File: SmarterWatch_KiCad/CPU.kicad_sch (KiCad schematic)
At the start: 14 parts, among them SW1 SW_SPST, SW2 SW_SPST, U5 ESP32-C6-MINI-1

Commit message: Button Footprint
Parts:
- SW1, SW2: footprint Smarter watching stuff foot:Button_smd_spst -> Custom_Foot:SMD_Button_6mm_SPST
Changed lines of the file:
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@@
 			)
 		)
-		(property "Footprint" "Smarter watching stuff foot:Button_smd_spst"
+		(property "Footprint" "Custom_Foot:SMD_Button_6mm_SPST"
 			(at 101.6 110.49 0)
 			(effects
@@
 			)
 		)
-		(property "Footprint" "Smarter watching stuff foot:Button_smd_spst"
+		(property "Footprint" "Custom_Foot:SMD_Button_6mm_SPST"
 			(at 82.55 81.28 0)
 			(effects

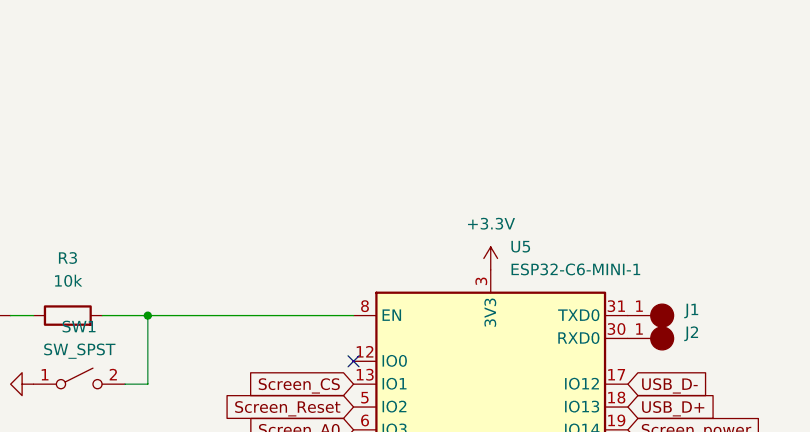
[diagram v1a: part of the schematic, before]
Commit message: more prgrs
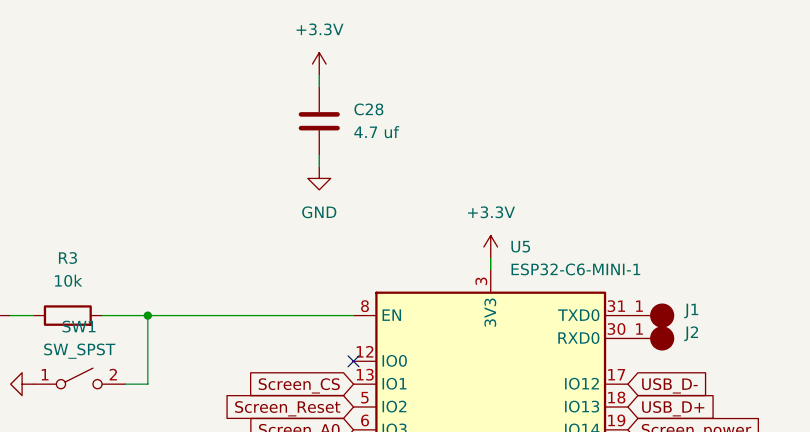
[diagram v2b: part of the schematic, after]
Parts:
- added C28: 4.7 uf, Capacitor_SMD:C_0402_1005Metric, symbol Device:C
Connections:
- net +3.3V: now also C28.1
- net GND: now also C28.2
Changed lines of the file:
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@@
+	(wire
+		(pts
+			(xy 128.27 67.31) (xy 128.27 68.58)
+		)
+		(stroke
+			(width 0)
+			(type default)
+		)
+	)
 	(wire
 		(pts
@@
 	(wire
 		(pts
-			(xy 113.03 96.52) (xy 110.49 96.52)
+			(xy 109.22 46.99) (xy 109.22 48.26)
 		)
 		(stroke
@@
 	(wire
 		(pts
-			(xy 87.63 81.28) (xy 90.17 81.28)
+			(xy 113.03 96.52) (xy 110.49 96.52)
 		)
 		(stroke
@@
 	(wire
 		(pts
-			(xy 111.76 101.6) (xy 111.76 110.49)
+			(xy 87.63 81.28) (xy 90.17 81.28)
 		)
 		(stroke
@@
 	(wire
 		(pts
-			(xy 85.09 73.66) (xy 90.17 73.66)
+			(xy 111.76 101.6) (xy 111.76 110.49)
 		)
 		(stroke
@@
 	(wire
 		(pts
-			(xy 104.14 101.6) (xy 111.76 101.6)
+			(xy 85.09 73.66) (xy 90.17 73.66)
 		)
 		(stroke
@@
 	(wire
 		(pts
-			(xy 93.98 99.06) (xy 96.52 99.06)
+			(xy 104.14 101.6) (xy 111.76 101.6)
 		)
 		(stroke
@@
 	(wire
 		(pts
-			(xy 106.68 110.49) (xy 111.76 110.49)
+			(xy 109.22 57.15) (xy 109.22 55.88)
 		)
 		(stroke
@@
 		)
 	)
+	(wire
+		(pts
+			(xy 93.98 99.06) (xy 96.52 99.06)
+		)
+		(stroke
+			(width 0)
+			(type default)
+		)
+	)
+	(wire
+		(pts
+			(xy 106.68 110.49) (xy 111.76 110.49)
+		)
+		(stroke
+			(width 0)
+			(type default)
+		)
+	)
 	(global_label "Screen_power"
 		(shape input)
@@
 	(symbol
 		(lib_id "power:+3.3V")
+		(at 109.22 46.99 0)
+		(unit 1)
+		(exclude_from_sim no)
+		(in_bom yes)
+		(on_board yes)
+		(dnp no)
+		(fields_autoplaced yes)
+		(property "Reference" "#PWR082"
+			(at 109.22 50.8 0)
+			(effects
+				(font
+					(size 1.27 1.27)
+				)
+				(hide yes)
+			)
+		)
+		(property "Value" "+3.3V"
+			(at 109.22 41.91 0)
+			(effects
+				(font
+					(size 1.27 1.27)
+				)
+			)
+		)
+		(property "Footprint" ""
+			(at 109.22 46.99 0)
+			(effects
+				(font
+					(size 1.27 1.27)
+				)
+				(hide yes)
+			)
+		)
+		(property "Datasheet" ""
+			(at 109.22 46.99 0)
+			(effects
+				(font
+					(size 1.27 1.27)
+				)
+				(hide yes)
+			)
+		)
+		(property "Description" "Power symbol creates a global label with name \"+3.3V\""
+			(at 109.22 46.99 0)
+			(effects
+				(font
+					(size 1.27 1.27)
+				)
+				(hide yes)
+			)
+		)
+		(pin "1"
+		)
+		(instances
+			(project "Smarter Watch Stuff"
+				(path "/52181fb0-1be8-41da-83b2-7d5a62778ff4/a00a754a-aed5-4908-97a0-bc1d443d4203"
+					(reference "#PWR082")
+					(unit 1)
+				)
+			)
+		)
+	)
+	(symbol
+		(lib_id "Device:C")
+		(at 109.22 52.07 0)
+		(unit 1)
+		(exclude_from_sim no)
+		(in_bom yes)
+		(on_board yes)
+		(dnp no)
+		(fields_autoplaced yes)
+		(property "Reference" "C28"
+			(at 113.03 50.7999 0)
+			(effects
+				(font
+					(size 1.27 1.27)
+				)
+				(justify left)
+			)
+		)
+		(property "Value" "4.7 uf"
+			(at 113.03 53.3399 0)
+			(effects
+				(font
+					(size 1.27 1.27)
+				)
+				(justify left)
+			)
+		)
+		(property "Footprint" "Capacitor_SMD:C_0402_1005Metric"
+			(at 110.1852 55.88 0)
+			(effects
+				(font
+					(size 1.27 1.27)
+				)
+				(hide yes)
+			)
+		)
+		(property "Datasheet" "~"
+			(at 109.22 52.07 0)
+			(effects
+				(font
+					(size 1.27 1.27)
+				)
+				(hide yes)
+			)
+		)
+		(property "Description" "Unpolarized capacitor"
+			(at 109.22 52.07 0)
+			(effects
+				(font
+					(size 1.27 1.27)
+				)
+				(hide yes)
+			)
+		)
+		(pin "1"
+		)
+		(pin "2"
+		)
+		(instances
+			(project "Smarter Watch Stuff"
+				(path "/52181fb0-1be8-41da-83b2-7d5a62778ff4/a00a754a-aed5-4908-97a0-bc1d443d4203"
+					(reference "C28")
+					(unit 1)
+				)
+			)
+		)
+	)
+	(symbol
+		(lib_id "power:+3.3V")
 		(at 93.98 101.6 90)
 		(unit 1)
@@
 	)
 	(symbol
+		(lib_id "power:GND")
+		(at 109.22 57.15 0)
+		(unit 1)
+		(exclude_from_sim no)
+		(in_bom yes)
+		(on_board yes)
+		(dnp no)
+		(fields_autoplaced yes)
+		(property "Reference" "#PWR0106"
+			(at 109.22 63.5 0)
+			(effects
+				(font
+					(size 1.27 1.27)
+				)
+				(hide yes)
+			)
+		)
+		(property "Value" "GND"
+			(at 109.22 62.23 0)
+			(effects
+				(font
+					(size 1.27 1.27)
+				)
+			)
+		)
+		(property "Footprint" ""
+			(at 109.22 57.15 0)
+			(effects
+				(font
+					(size 1.27 1.27)
+				)
+				(hide yes)
+			)
+		)
+		(property "Datasheet" ""
+			(at 109.22 57.15 0)
+			(effects
+				(font
+					(size 1.27 1.27)
+				)
+				(hide yes)
+			)
+		)
+		(property "Description" "Power symbol creates a global label with name \"GND\" , ground"
+			(at 109.22 57.15 0)
+			(effects
+				(font
+					(size 1.27 1.27)
+				)
+				(hide yes)
+			)
+		)
+		(pin "1"
+		)
+		(instances
+			(project "Smarter Watch Stuff"
+				(path "/52181fb0-1be8-41da-83b2-7d5a62778ff4/a00a754a-aed5-4908-97a0-bc1d443d4203"
+					(reference "#PWR0106")
+					(unit 1)
+				)
+			)
+		)
+	)
+	(symbol
 		(lib_id "Switch:SW_SPST")
 		(at 82.55 81.28 0)
@@
 	(symbol
 		(lib_id "power:+3.3V")
-		(at 128.27 68.58 0)
+		(at 128.27 67.31 0)
 		(unit 1)
 		(exclude_from_sim no)
@@
 		(fields_autoplaced yes)
 		(property "Reference" "#PWR020"
-			(at 128.27 72.39 0)
+			(at 128.27 71.12 0)
 			(effects
 				(font
@@
 		)
 		(property "Value" "+3.3V"
-			(at 128.27 63.5 0)
+			(at 128.27 62.23 0)
 			(effects
 				(font
@@
 		)
 		(property "Footprint" ""
-			(at 128.27 68.58 0)
+			(at 128.27 67.31 0)
 			(effects
 				(font
@@
 		)
 		(property "Datasheet" ""
-			(at 128.27 68.58 0)
+			(at 128.27 67.31 0)
 			(effects
 				(font
@@
 		)
 		(property "Description" "Power symbol creates a global label with name \"+3.3V\""
-			(at 128.27 68.58 0)
-			(effects
-				(font
+			(at 128.27 67.31 0)
+			(effects
+				(font

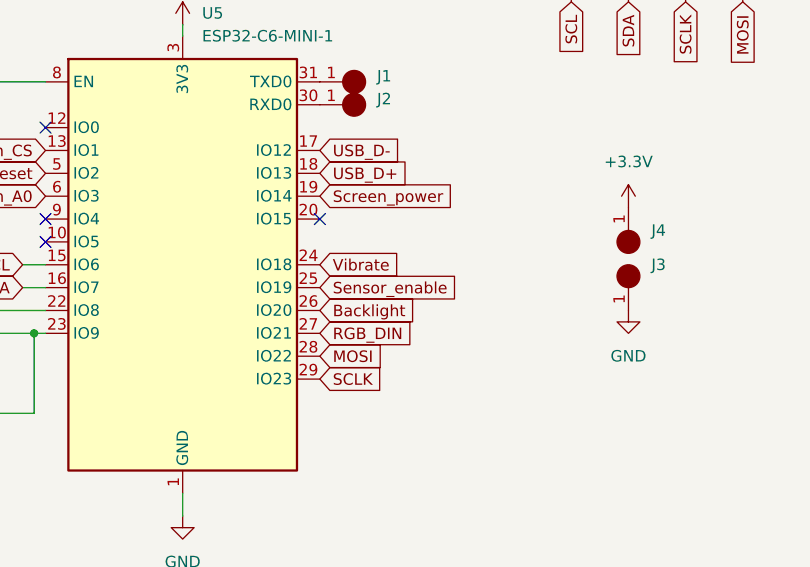
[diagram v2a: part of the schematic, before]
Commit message: Yay!
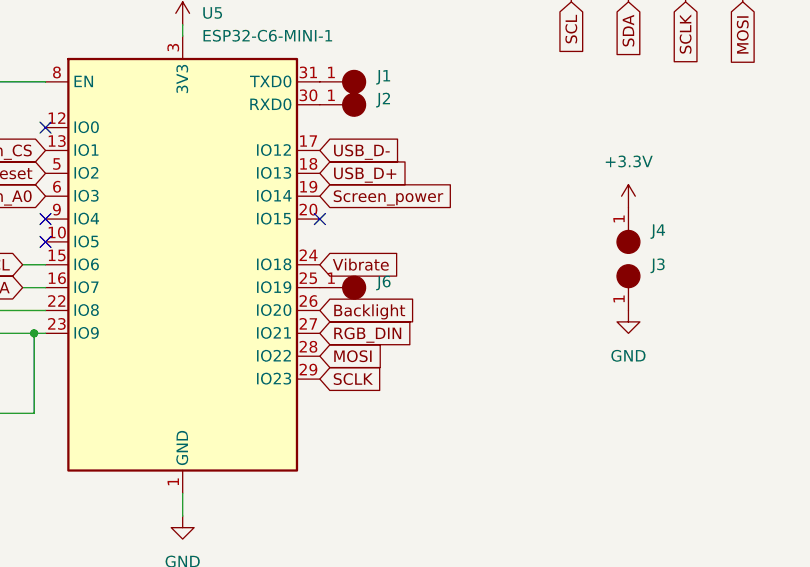
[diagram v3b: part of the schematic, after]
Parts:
- added J6: ~, Connector_Wire:SolderWirePad_1x01_SMD_2x4mm, symbol SmarterWatch_symbols_j:Solder_pad
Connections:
- net Sensor_enable: no longer names the net of U5.25 (IO19)
- net Sensor_enable: now also J6.1
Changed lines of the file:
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@@
 		)
 	)
-	(global_label "Sensor_enable"
+	(global_label "SCL"
 		(shape input)
-		(at 143.51 96.52 0)
+		(at 110.49 93.98 180)
 		(fields_autoplaced yes)
 		(effects
@@
 				(size 1.27 1.27)
 			)
-			(justify left)
+			(justify right)
 		)
 		(property "Intersheetrefs" "${INTERSHEET_REFS}"
-			(at 160.1626 96.52 0)
-			(effects
-				(font
-					(size 1.27 1.27)
-				)
-				(justify left)
-				(hide yes)
-			)
-		)
-	)
-	(global_label "SCL"
+			(at 103.9972 93.98 0)
+			(effects
+				(font
+					(size 1.27 1.27)
+				)
+				(justify right)
+				(hide yes)
+			)
+		)
+	)
+	(global_label "SDA"
 		(shape input)
-		(at 110.49 93.98 180)
+		(at 110.49 96.52 180)
 		(fields_autoplaced yes)
 		(effects
@@
 		)
 		(property "Intersheetrefs" "${INTERSHEET_REFS}"
-			(at 103.9972 93.98 0)
+			(at 103.9367 96.52 0)
 			(effects
 				(font
@@
 		)
 	)
-	(global_label "SDA"
+	(global_label "Backlight"
 		(shape input)
-		(at 110.49 96.52 180)
+		(at 143.51 99.06 0)
 		(fields_autoplaced yes)
 		(effects
@@
 				(size 1.27 1.27)
 			)
-			(justify right)
+			(justify left)
 		)
 		(property "Intersheetrefs" "${INTERSHEET_REFS}"
-			(at 103.9367 96.52 0)
-			(effects
-				(font
-					(size 1.27 1.27)
-				)
-				(justify right)
-				(hide yes)
-			)
-		)
-	)
-	(global_label "Backlight"
+			(at 155.3246 99.06 0)
+			(effects
+				(font
+					(size 1.27 1.27)
+				)
+				(justify left)
+				(hide yes)
+			)
+		)
+	)
+	(global_label "SDA"
 		(shape input)
-		(at 143.51 99.06 0)
+		(at 177.8 64.77 270)
 		(fields_autoplaced yes)
 		(effects
@@
 				(size 1.27 1.27)
 			)
-			(justify left)
+			(justify right)
 		)
 		(property "Intersheetrefs" "${INTERSHEET_REFS}"
-			(at 155.3246 99.06 0)
-			(effects
-				(font
-					(size 1.27 1.27)
-				)
-				(justify left)
-				(hide yes)
-			)
-		)
-	)
-	(global_label "SDA"
+			(at 177.8 71.3233 90)
+			(effects
+				(font
+					(size 1.27 1.27)
+				)
+				(justify right)
+				(hide yes)
+			)
+		)
+	)
+	(global_label "Screen_Reset"
 		(shape input)
-		(at 177.8 64.77 270)
+		(at 113.03 83.82 180)
 		(fields_autoplaced yes)
 		(effects
@@
 		)
 		(property "Intersheetrefs" "${INTERSHEET_REFS}"
-			(at 177.8 71.3233 90)
-			(effects
-				(font
-					(size 1.27 1.27)
-				)
-				(justify right)
-				(hide yes)
-			)
-		)
-	)
-	(global_label "Screen_Reset"
-		(shape input)
-		(at 113.03 83.82 180)
-		(fields_autoplaced yes)
-		(effects
-			(font
-				(size 1.27 1.27)
-			)
-			(justify right)
-		)
-		(property "Intersheetrefs" "${INTERSHEET_REFS}"
 			(at 97.4657 83.82 0)
 			(effects
@@
 					(unit 1)
 				)
+			)
+		)
+	)
+	(symbol
+		(lib_name "Solder_pad_1")
+		(lib_id "SmarterWatch_symbols_j:Solder_pad")
+		(at 147.32 93.98 0)
+		(unit 1)
+		(exclude_from_sim no)
+		(in_bom yes)
+		(on_board yes)
+		(dnp no)
+		(fields_autoplaced yes)
+		(property "Reference" "J6"
+			(at 149.86 95.8849 0)
+			(effects
+				(font
+					(size 1.27 1.27)
+				)
+				(justify left)
+			)
+		)
+		(property "Value" "~"
+			(at 149.86 97.79 0)
+			(effects
+				(font
+					(size 1.27 1.27)
+				)
+				(justify left)
+			)
+		)
+		(property "Footprint" "Connector_Wire:SolderWirePad_1x01_SMD_2x4mm"
+			(at 147.32 93.98 0)
+			(effects
+				(font
+					(size 1.27 1.27)
+				)
+				(hide yes)
+			)
+		)
+		(property "Datasheet" ""
+			(at 147.32 93.98 0)
+			(effects
+				(font
+					(size 1.27 1.27)
+				)
+				(hide yes)
+			)
+		)
+		(property "Description" ""
+			(at 147.32 93.98 0)
+			(effects
+				(font
+					(size 1.27 1.27)
+				)
+				(hide yes)
+			)
+		)
+		(pin "1"
+		)
+		(instances
+			(project "Smarter Watch Stuff"
+				(path "/52181fb0-1be8-41da-83b2-7d5a62778ff4/a00a754a-aed5-4908-97a0-bc1d443d4203"
+					(reference "J6")
+					(unit 1)
+				)

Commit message: FINAL
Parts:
- J1, J2, J3, J4, J6: value ~ -> (none)
